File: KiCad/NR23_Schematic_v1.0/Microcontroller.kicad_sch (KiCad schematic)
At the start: 19 parts

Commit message: start of class 26apr23
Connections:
- new net: U?. (GND), U?. (To_TI_CAN_L) (x2)

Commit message: endof day 26APR23
changed the wires going into the ti board box in order to match what is actually on the car
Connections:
- new net: U?. (GND), U?. (To_TI_CAN_L) (x2)

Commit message: end of class on 01APR23 - battery stuff
Added new battery connections and reprinted battery schematic
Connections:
- new net: U?. (GND), U?. (To_TI_CAN_L) (x2)

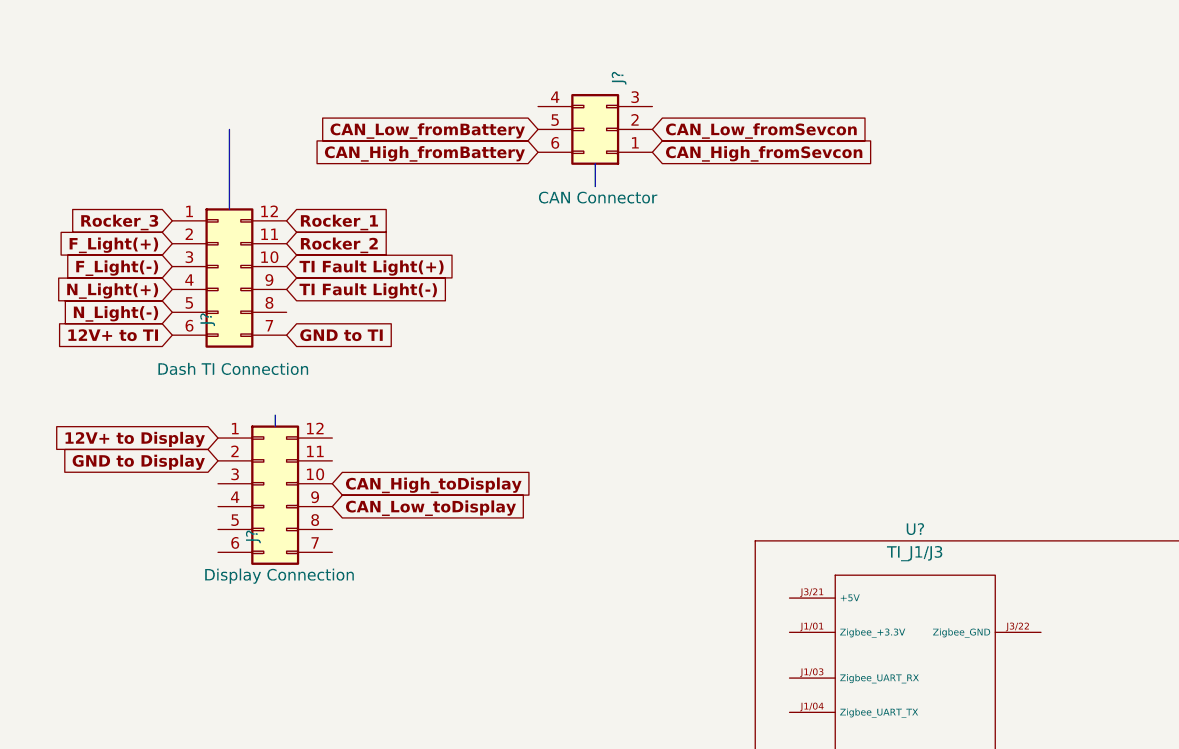
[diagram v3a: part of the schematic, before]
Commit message: end of day 02APR23
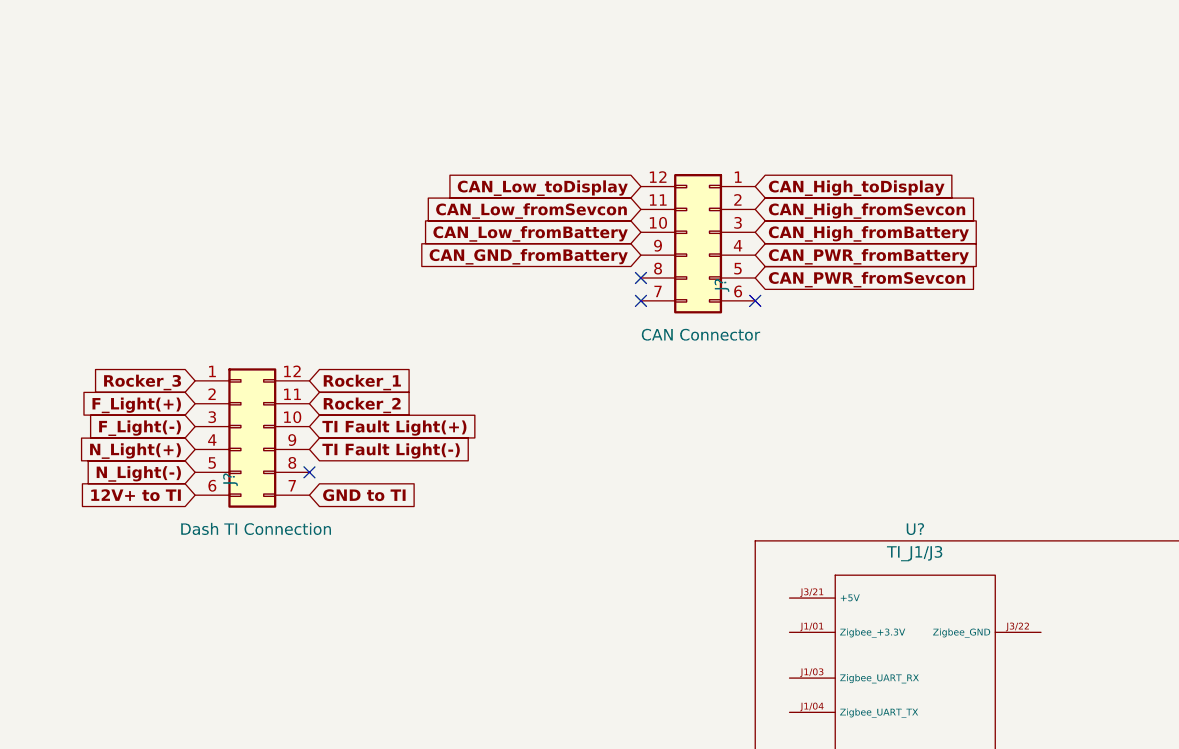
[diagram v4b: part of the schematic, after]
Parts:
- removed J?: Display Connection, symbol Connector_Generic:Conn_02x06_Counter_Clockwise
- removed J?: Dash TI Connection, symbol Connector_Generic:Conn_02x06_Counter_Clockwise
- removed J?: CAN Connector, symbol Connector_Generic:Conn_02x03_Counter_Clockwise
- added J?: Dash TI Connection, symbol Connector_Generic:Conn_02x06_Counter_Clockwise
- added J?: CAN Connector, symbol Connector_Generic:Conn_02x06_Counter_Clockwise
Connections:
- net 12V+ to TI: now also J?.6 (Pin_6)
- net CAN_High_fromBattery: now also J?.3 (Pin_3)
- net CAN_High_fromSevcon: now also J?.2 (Pin_2)
- net CAN_High_toDisplay: now also J?.1 (Pin_1)
- net CAN_Low_fromBattery: now also J?.10 (Pin_10)
- net CAN_Low_fromSevcon: now also J?.11 (Pin_11)
- net CAN_Low_toDisplay: now also J?.12 (Pin_12)
- net F_Light(+): now also J?.2 (Pin_2)
- net F_Light(-): now also J?.3 (Pin_3)
- net GND to TI: now also J?.7 (Pin_7)
- net N_Light(+): now also J?.4 (Pin_4)
- net N_Light(-): now also J?.5 (Pin_5)
- net Rocker_1: now also J?.12 (Pin_12)
- net Rocker_2: now also J?.11 (Pin_11)
- net Rocker_3: now also J?.1 (Pin_1)
- net TI Fault Light(+): now also J?.10 (Pin_10)
- net TI Fault Light(-): now also J?.9 (Pin_9)
- new net: U?. (GND), U?. (To_TI_CAN_L) (x2)
- new net CAN_GND_fromBattery: J?.9 (Pin_9)
- new net CAN_PWR_fromBattery: J?.4 (Pin_4)
- new net CAN_PWR_fromSevcon: J?.5 (Pin_5)
- no-connect marks 0 -> 4
